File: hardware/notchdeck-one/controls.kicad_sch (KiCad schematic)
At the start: 38 parts, among them SW1 SW_Push, SW10 SW_Push, SW11 SW_Push, SW12 SW_Push, SW13 SW_Push, SW14 SW_Push, SW15 SW_Push, SW16 SW_Push, SW2 SW_Push, SW3 SW_Push, SW4 SW_Push, SW5 SW_Push, SW6 SW_Push, SW7 SW_Push, SW8 SW_Push, SW9 SW_Push

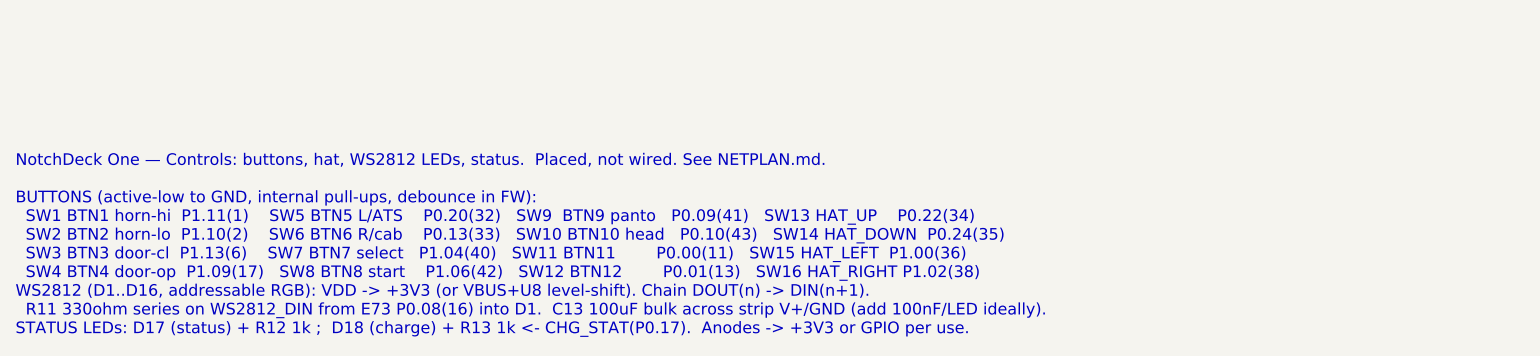
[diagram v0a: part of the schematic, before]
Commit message: Add schematic wiring notes support
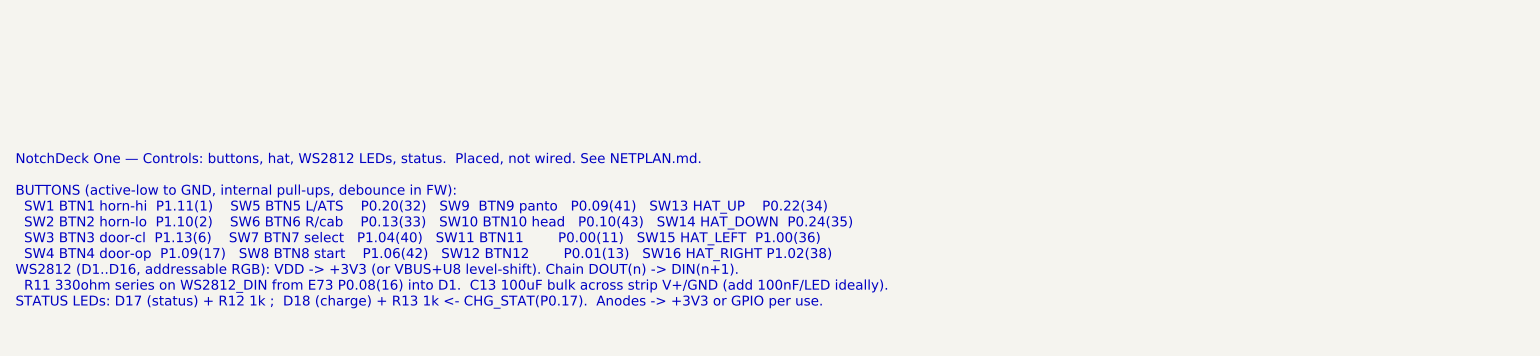
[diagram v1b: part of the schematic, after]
